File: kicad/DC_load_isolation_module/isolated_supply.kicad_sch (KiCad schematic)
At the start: 43 parts, among them Q10 AO3400A, Q11 AO3400A, Q12 MMBT5551L, Q14 MMBT5401, Q15 MMBT5551L, Q16 MMBT5551L, Q8 MMBT5551L, Q9 MMBT5401

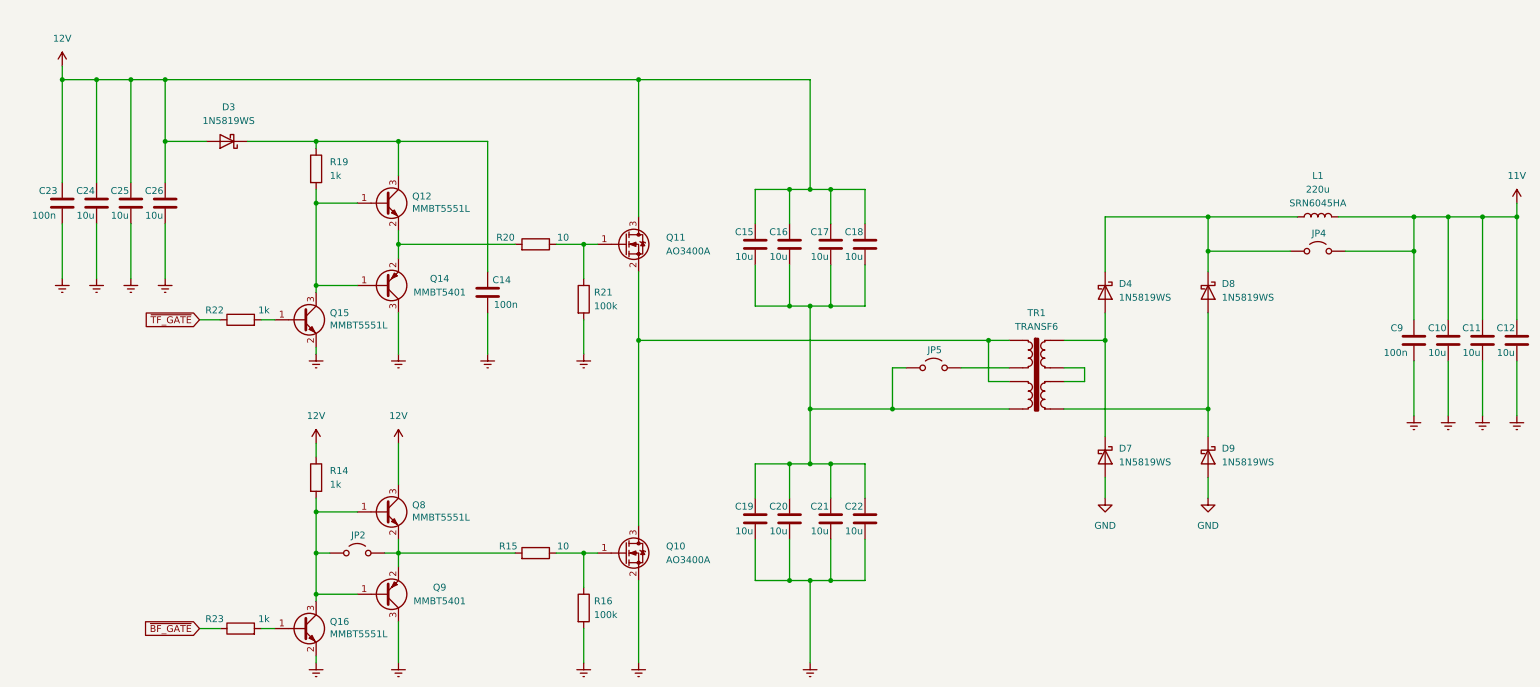
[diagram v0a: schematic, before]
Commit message: Idk.
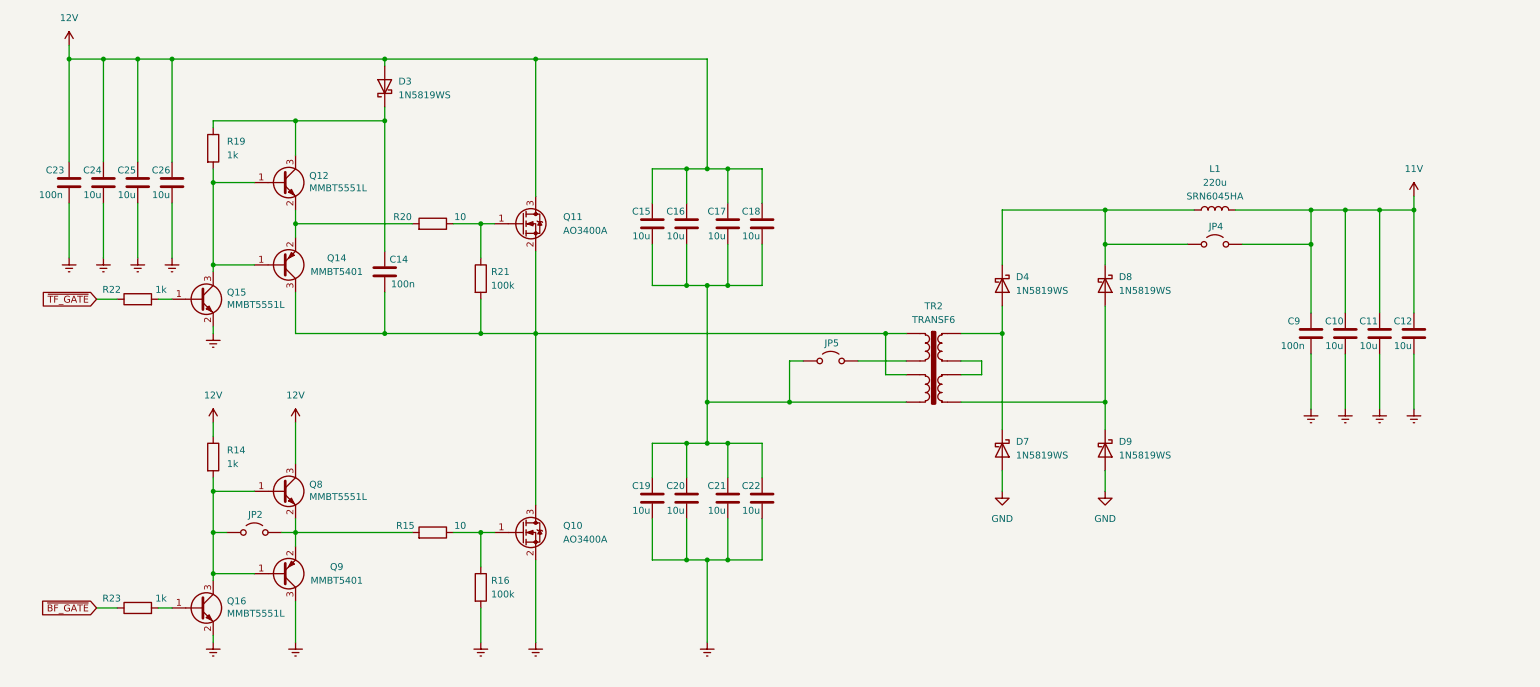
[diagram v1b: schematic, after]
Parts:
- renumbered TR1 to TR2
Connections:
- net Earth: no longer C14.2, Q14.3 (C), R21.2
- net at Q10.3 (D), Q11.2 (S), TR2.1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: now also C14.2, Q14.3 (C), R21.2
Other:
- moved on the sheet: C10, C11, C12, C14, C15, C16, C17, C18, C19, C20, C21, C22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
